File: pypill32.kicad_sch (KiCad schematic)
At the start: 37 parts, among them J1 HeaderR, J2 HeaderL, J4 ISP, SW1 SW_Push, SW2 SW_Push, U1 SRV05-4, U2 PY32F030F18P6, U3 CH340N

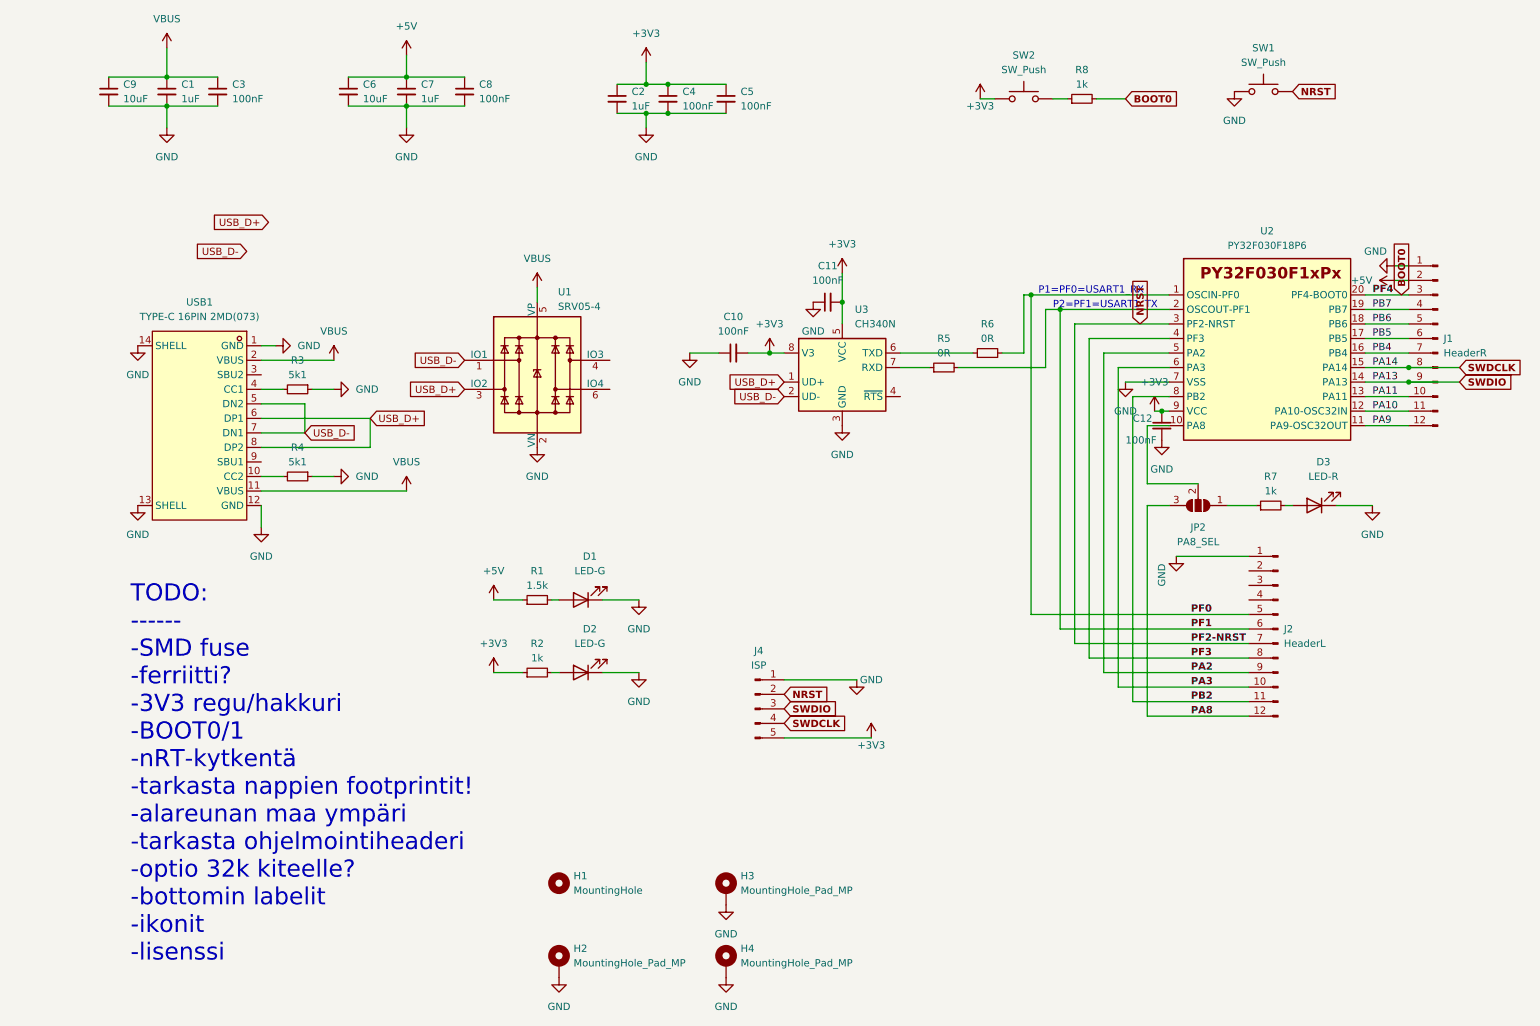
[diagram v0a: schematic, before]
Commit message: some progress
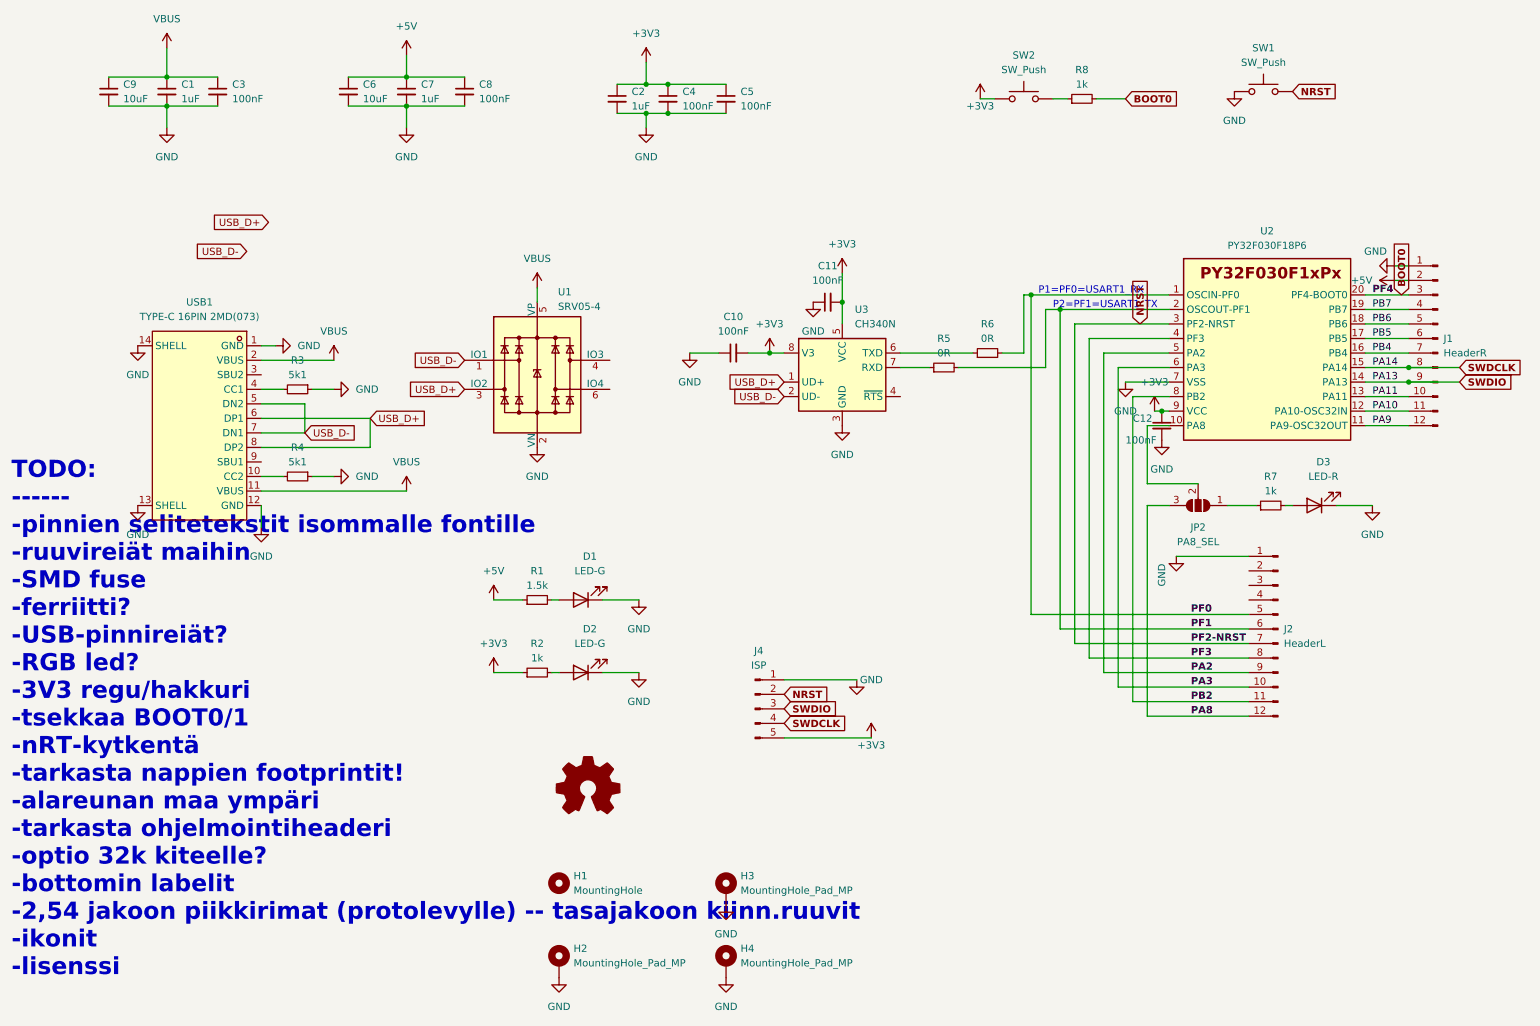
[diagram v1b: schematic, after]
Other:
- note added: "TODO: ------ -pinnien selitetekstit isommalle fontille -ruuvireiät maihin -SMD fuse -ferriitti? -USB-pinnireiät? -RGB led? -3V3 regu/hakkuri -tsekkaa BOOT0/1 -nRT-kytkentä -tarkasta nappien footprintit! -alareunan maa ympäri -tarkasta ohjelmointiheaderi -optio 32k kiteelle? -bottomin labelit -2,54 jakoon piikkirimat (protolevylle) -- tasajakoon kiinn.ruuvit -ikonit -lisenssi"
- note removed: "TODO: ------ -SMD fuse -ferriitti? -3V3 regu/hakkuri -BOOT0/1 -nRT-kytkentä -tarkasta nappien footprintit! -alareunan maa ympäri -tarkasta ohjelmointiheaderi -optio 32k kiteelle? -bottomin labelit -ikonit -lisenssi"
